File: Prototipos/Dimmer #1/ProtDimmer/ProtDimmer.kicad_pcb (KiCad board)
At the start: 2 copper layers, 114.3 x 83.8 mm, 22 parts, among them J1 Conn_01x02, J2 Conn_01x02, J3 Conn_01x05, K1 SRD-05VDC-SL-C, Q1 BC548B, Q2 BT137, U1 MOC3021M, U2 EL817

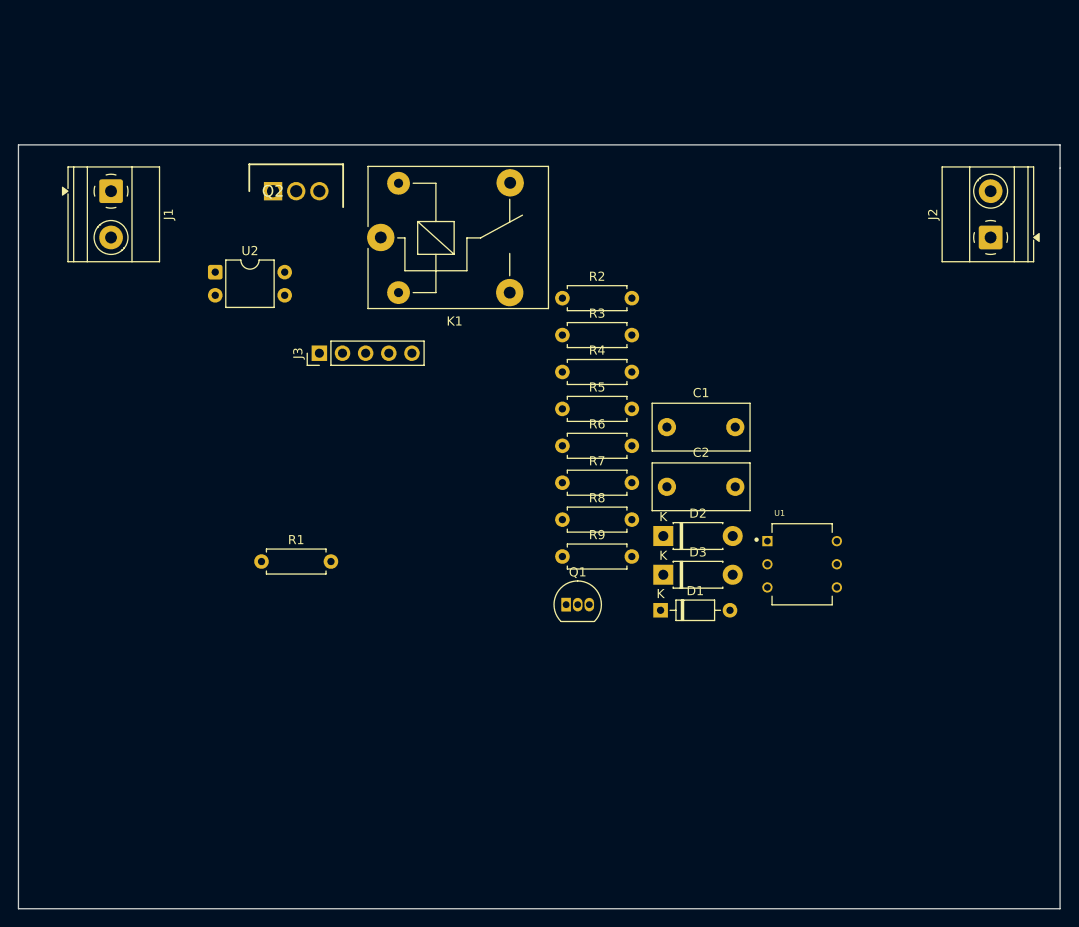
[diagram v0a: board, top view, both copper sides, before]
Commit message: Primera versión pcb
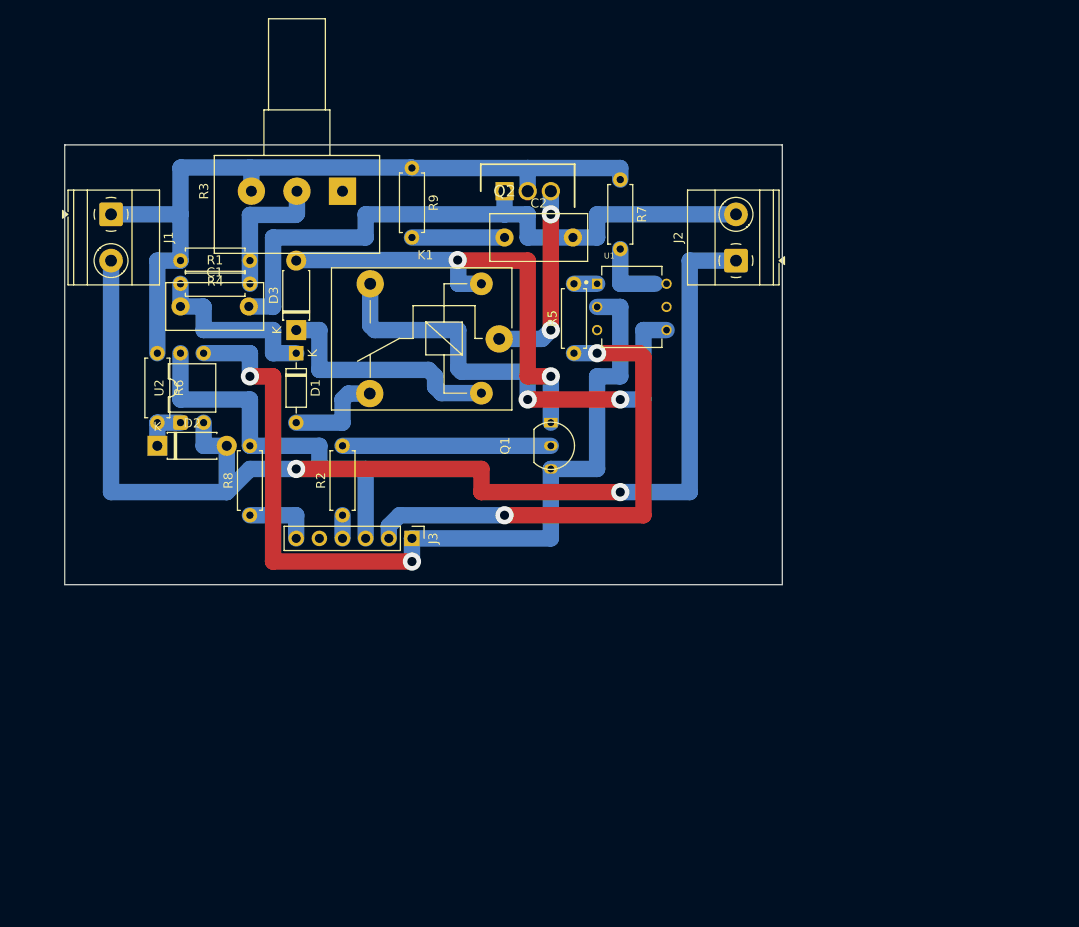
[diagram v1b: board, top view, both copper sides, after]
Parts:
- J3: footprint Connector_PinHeader_2.54mm:PinHeader_1x05_P2.54mm_Vertical -> Connector_PinHeader_2.54mm:PinHeader_1x06_P2.54mm_Vertical
- R3: footprint Resistor_THT:R_Axial_DIN0207_L6.3mm_D2.5mm_P7.62mm_Horizontal -> Potentiometer_THT:Potentiometer_Alps_RK163_Single_Horizontal
- moved D2 56.4 mm to (88.9, 78.7)
- moved C1 55.0 mm to (91.4, 63.5)
- moved D1 48.9 mm to (104.1, 68.6), turned to -90 degrees
- moved D3 48.4 mm to (104.1, 66.0), turned to 90 degrees
- moved R9 45.7 mm to (116.8, 48.3), turned to -90 degrees
- moved R6 45.6 mm to (88.9, 68.6), turned to -90 degrees
- moved R4 35.6 mm to (99.1, 61.0), turned to 180 degrees
- moved R8 34.3 mm to (99.1, 86.4), turned to 90 degrees
- moved R1 34.2 mm to (91.4, 58.4)
- moved R2 33.9 mm to (109.2, 86.4), turned to 90 degrees
- moved U1 33.9 mm to (141.0, 63.5)
- moved R7 33.9 mm to (139.7, 49.5), turned to -90 degrees
- moved C2 32.7 mm to (127.0, 55.9)
- moved R3 28.8 mm to (109.2, 50.8), turned to -90 degrees
- moved J2 28.1 mm to (152.4, 58.4)
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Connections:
- J2 pad 1: Load_N -> 48Vca_N
- J2 pad 2: Load_L -> LOAD_L
- J3 pad 2: UC_PHASE -> UC_DOUT
- J3 pad 3: UC_RELAY -> UC_PHASE
- J3 pad 4: 3.3Vcc -> UC_RELAY
- R3 pad 1: 48Vca_L -> (no net)
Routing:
- net 48Vca_N: track 0.00 -> 133.1 mm, vias 0 -> 2
- net GND: track 0.00 -> 99.1 mm, vias 0 -> 2
- net 48Vca_L: track 0.00 -> 85.3 mm
- net LOAD_L: track 0.00 -> 71.3 mm
- net UC_DOUT: track 0.00 -> 54.9 mm, vias 0 -> 2
- net Net-(K1-Pad3): track 0.00 -> 52.0 mm, vias 0 -> 2
- net RELAY_T2: track 0.00 -> 50.9 mm, vias 0 -> 2
- net UC_PHASE: track 0.00 -> 40.6 mm
- net 5Vcc: track 0.00 -> 26.4 mm
- net Net-(Q1-B): track 0.00 -> 22.9 mm
- net Net-(Q2-G): track 0.00 -> 21.7 mm, vias 0 -> 2
- net Net-(D1-K): track 0.00 -> 20.3 mm
- net Net-(R1-Pad2): track 0.00 -> 15.2 mm
- net Net-(D1-A): track 0.00 -> 10.9 mm
- net Net-(C2-Pad1): track 0.00 -> 10.2 mm
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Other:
- board size 114.3 x 83.8 mm -> 78.7 x 48.3 mm
